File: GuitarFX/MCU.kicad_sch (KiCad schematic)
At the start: 43 parts, among them J301 USB_C_Receptacle_USB2.0, J302 Conn_ARM_SWD_TagConnect_TC2030, J303 Screw_Terminal_01x06, SW301 SW_SPDT, U2 STM32H733VGTx, U301 USBLC6-2SC6, Y301 24MHz

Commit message: Finished rough layout for MCU
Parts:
- C302: footprint Capacitor_SMD:C_0603_1608Metric -> Capacitor_SMD:C_0402_1005Metric

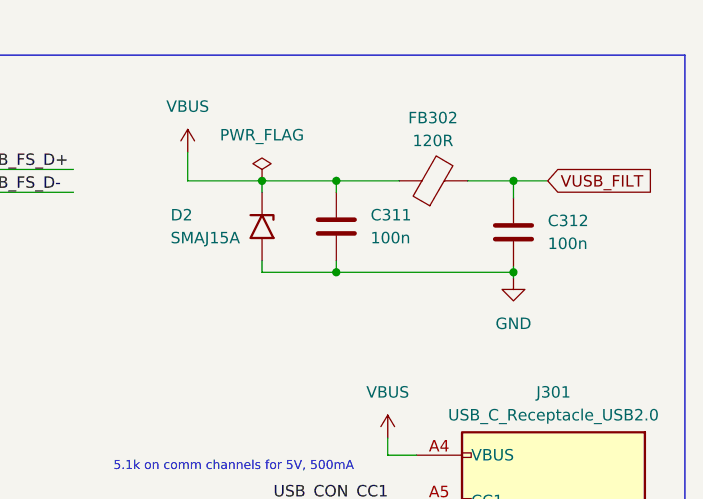
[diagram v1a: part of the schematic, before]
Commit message: Finished rough layout
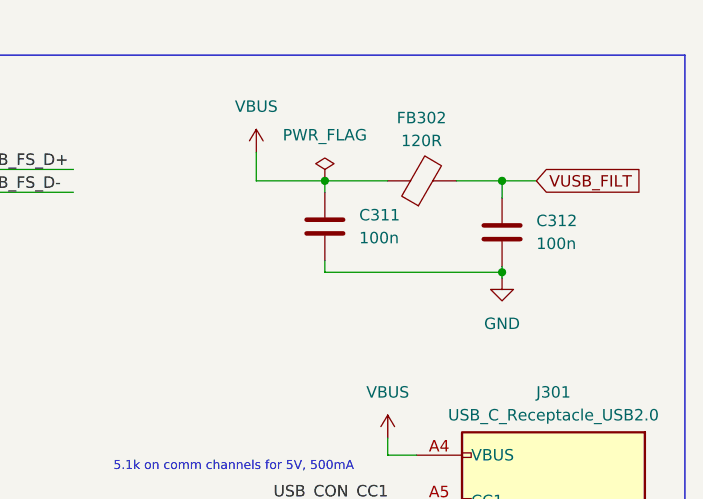
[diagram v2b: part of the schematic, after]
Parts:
- removed D2: SMAJ15A, Diode_SMD:D_SMA, symbol Diode:SMAJ15A
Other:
- moved on the sheet: C311, C312, FB302
